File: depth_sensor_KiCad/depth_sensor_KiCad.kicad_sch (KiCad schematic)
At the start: 11 parts, among them U1 RP2040, U10 DRV5055A3, U11 DRV5055A3, U2 DRV5055A3, U3 DRV5055A3, U4 DRV5055A3, U5 DRV5055A3, U6 SN74LV4051APWR, U8 DRV5055A3, U9 DRV5055A3

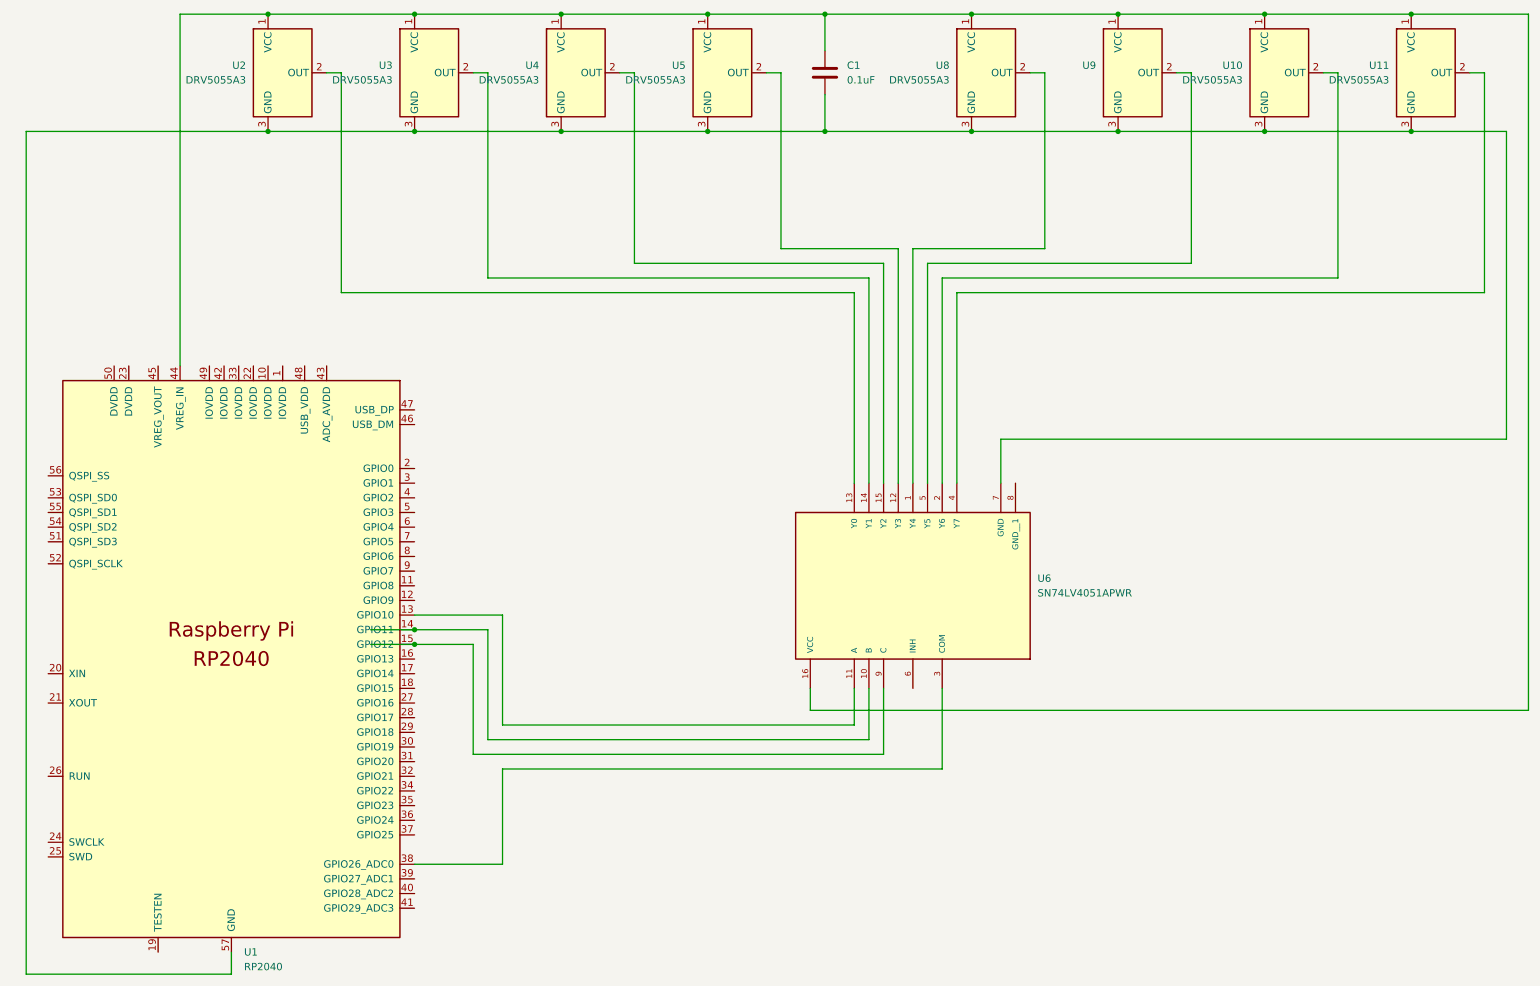
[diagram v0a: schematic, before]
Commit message: added latest changes
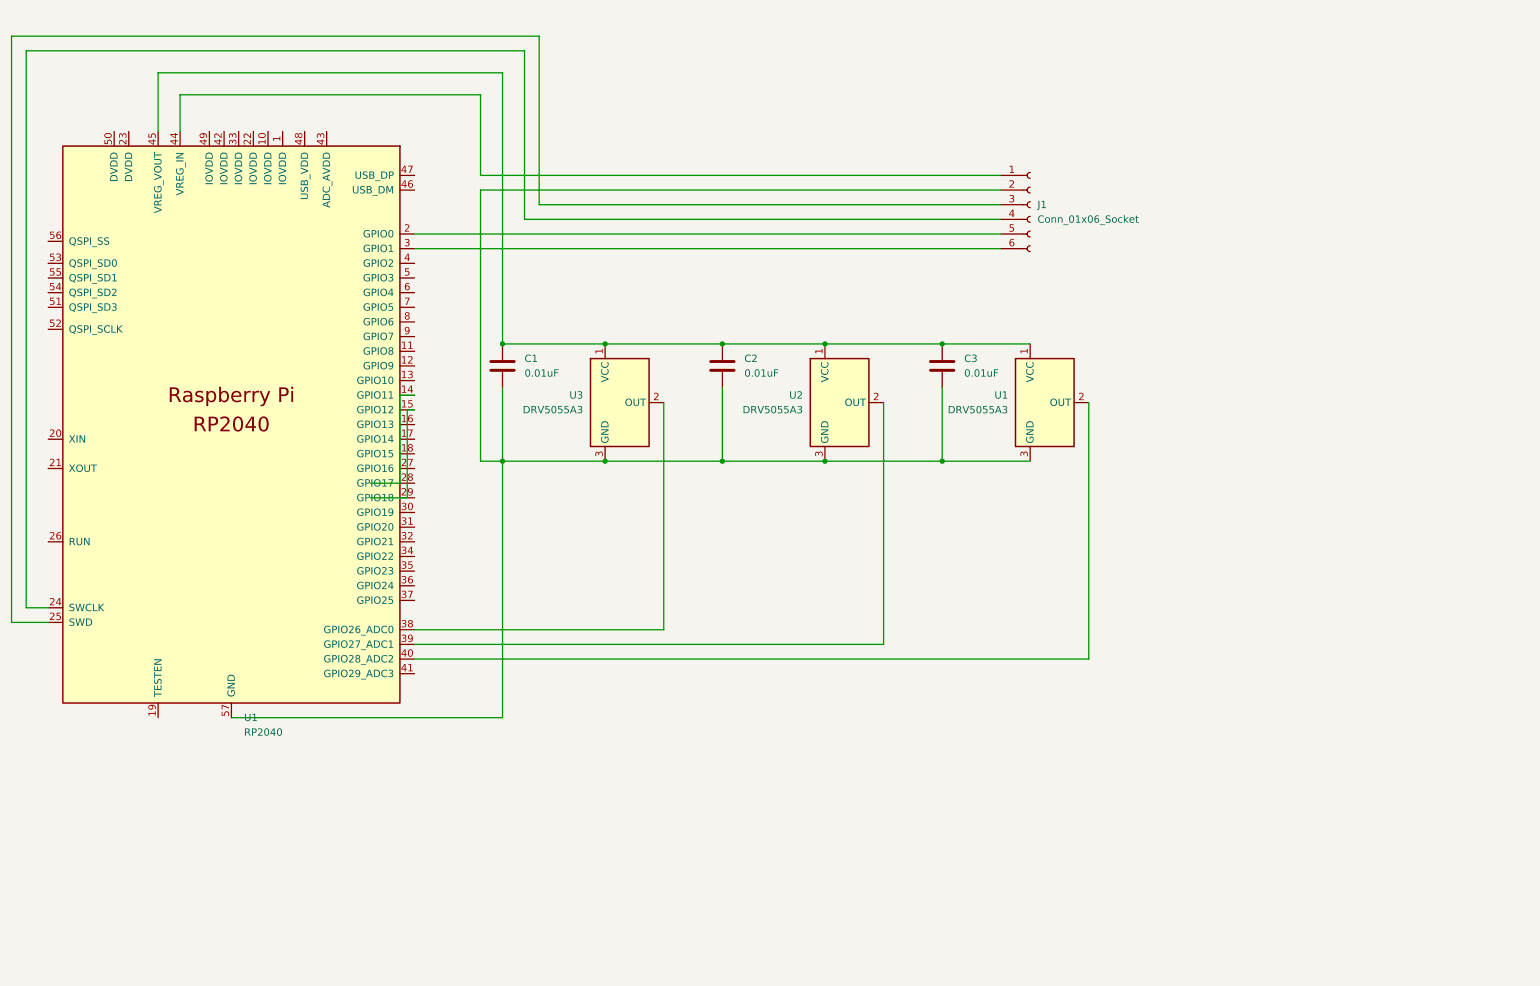
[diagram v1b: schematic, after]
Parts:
- removed U10, U11, U4, U5, U8, U9: DRV5055A3, Package_TO_SOT_SMD:SOT-23, symbol Sensor_Magnetic:DRV5055A3xDBZxQ1
- removed U6: SN74LV4051APWR, SN74LV4051APWR:SOP65P640X120-16N, symbol SN74LV4051APWR:SN74LV4051APWR
- added C1, C3: 0.01uF, symbol Device:C
- added J1: Conn_01x06_Socket, symbol Connector:Conn_01x06_Socket
- added U2: DRV5055A3, Package_TO_SOT_SMD:SOT-23, symbol Sensor_Magnetic:DRV5055A3xDBZxQ1
- C2: renamed from C1; value 0.1uF -> 0.01uF
- renumbered U2 to U1
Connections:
- net at C2.1, U1.1 (VCC), U3.1 (VCC): now also U1.45 (VREG_VOUT), C1.1, C3.1, U2.1 (VCC); no longer U1.44 (VREG_IN)
- net at C2.2, U1.3 (GND), U1.57 (GND)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: now also C1.2, C3.2, J1.2 (Pin_2), U2.3 (GND)
- net at U3.2 (OUT): now also U1.38 (GPIO26_ADC0)
- net at U1.2 (OUT): now also U1.40 (GPIO28_ADC2)
- net at U1.2 (GPIO0): now also J1.5 (Pin_5)
- net at U1.24 (SWCLK): now also J1.4 (Pin_4)
- net at U1.25 (SWD): now also J1.3 (Pin_3)
- net at U1.3 (GPIO1): now also J1.6 (Pin_6)
- net at U1.39 (GPIO27_ADC1): now also U2.2 (OUT)
- new net: J1.1 (Pin_1), U1.44 (VREG_IN)
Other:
- moved on the sheet: C2, U1
